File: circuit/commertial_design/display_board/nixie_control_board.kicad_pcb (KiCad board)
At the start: 2 copper layers, 200 x 63 mm, 12 parts, among them P1 CONN_02X01, P5 CONN_01X08, P6 CONN_01X12, SW3 SW_PUSH, U10 IN-14, U11 IN-14, U12 IN-14, U13 IN-14, U14 IN-14, U15 IN-14, U16 IN-14, U17 IN-14

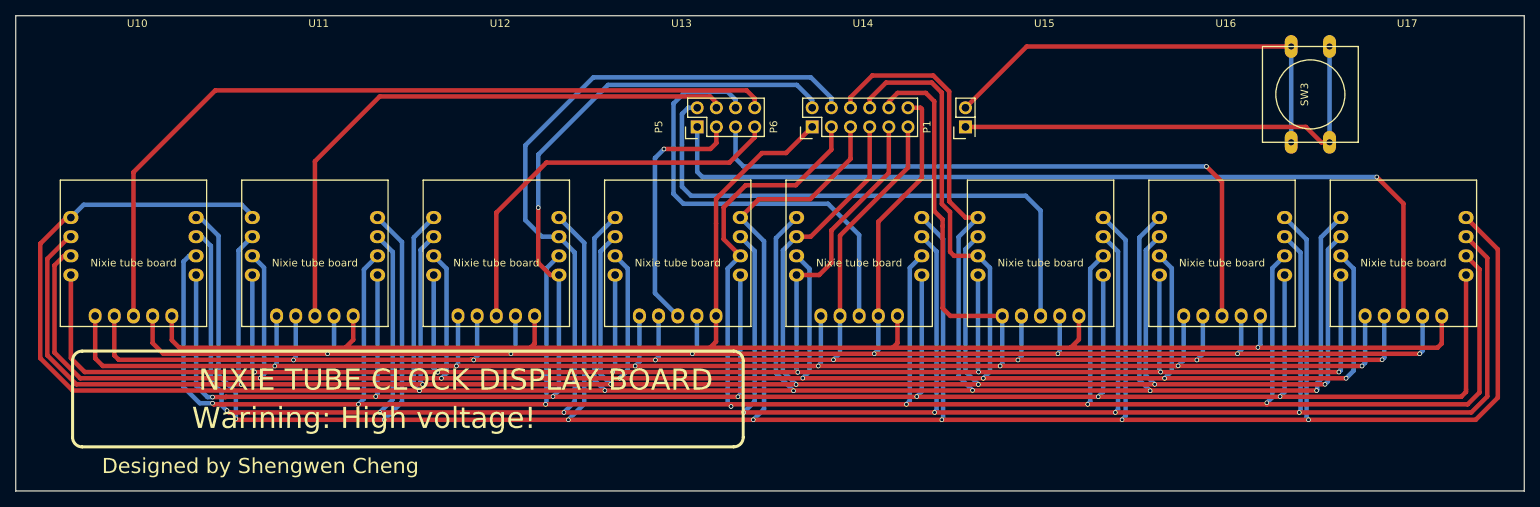
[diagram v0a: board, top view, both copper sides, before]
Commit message: Update commertial board
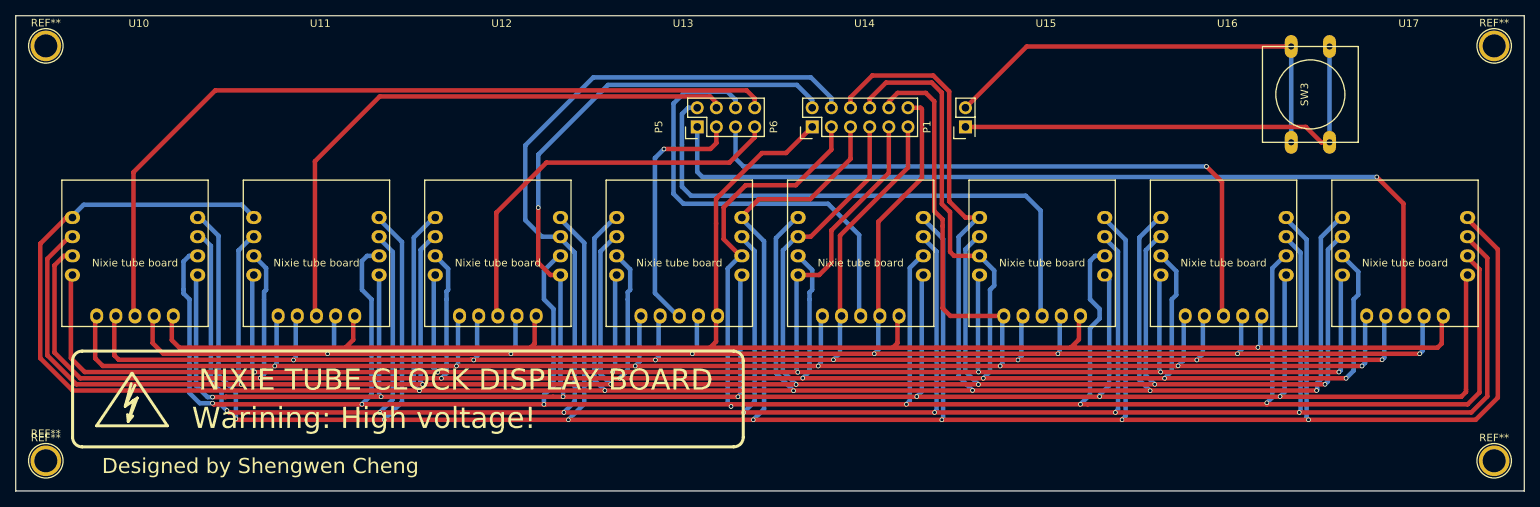
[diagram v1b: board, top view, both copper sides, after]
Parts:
- added REF**: 1pin, Connect:1pin, F.Cu at (248.1, 74.6)
- added REF**: 1pin, Connect:1pin, F.Cu at (248.1, 129.6)
- added REF**: 1pin, Connect:1pin, F.Cu at (56.1, 74.6)
- added REF**: 1pin, Connect:1pin, F.Cu at (56.1, 129.6)
- added REF**: Symbol_HighVoltage_Type2_CopperTop_VerySmall, warning:warning, F.Cu at (67.5, 122.1)
- added REF**: Symbol_HighVoltage_Type2_CopperTop_VerySmall, warning:warning, B.Cu at (67.5, 81.5)
- moved U14 0.21 mm to (164.1, 102.1)
- moved U15 0.21 mm to (188.1, 102.1)
- moved U17 0.21 mm to (236.2, 102.1)
- moved U10 0.20 mm to (67.9, 102.1)
- moved U11 0.20 mm to (91.9, 102.1)
- moved U12 0.20 mm to (116.0, 102.1)
- moved U13 0.20 mm to (140.0, 102.1)
- moved U16 0.20 mm to (212.2, 102.1)
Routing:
- net cathode8: track 362.6 -> 368.1 mm
- net cathode3: track 345.9 -> 347.7 mm
- net cathode9: track 357.3 -> 358.0 mm
